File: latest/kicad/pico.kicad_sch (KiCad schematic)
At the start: 69 parts, among them J1 Jack 3.5mm, J12 Debug, J14 JST PH 4, J2 DIN5, J25 JST PH 3, J26 JST PH 3, J3 Jack 3.5mm, J4 DIN5, J5 Jack 6.35mm, J8 Jack 6.35mm, SW1 24P/R 24mm, SW10 Tactile Button, SW2 24P/R 24mm, SW3 Micro Button, SW4 Micro Button, SW5 Tactile Button, SW6 Tactile Button, SW7 Tactile Button, SW8 Tactile Button, SW9 Tactile Button, U12 AT24CS01-STUM, U2 TLP2761, U3 RP2040, U4 W25Q128JVS, Y2 ABM8-272-T3

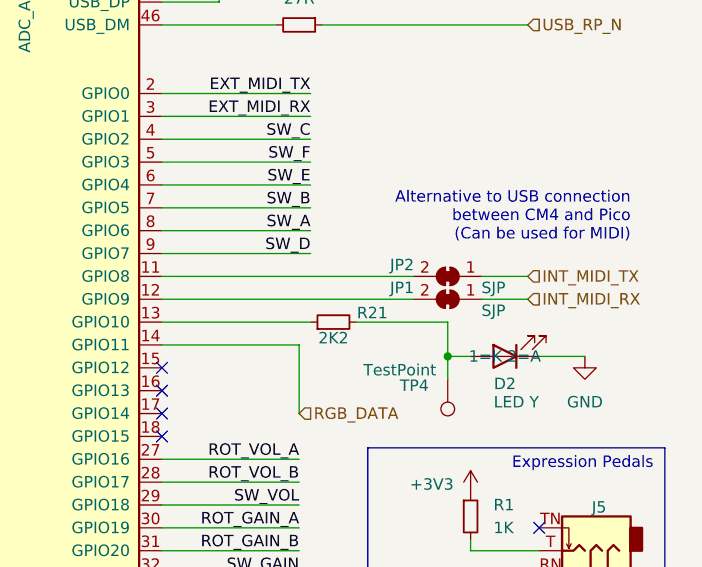
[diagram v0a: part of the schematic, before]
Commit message: Deploying to gh-pages from @ pedalboard/pedalboard-hw@99058ce3b2bc7db122aa04b2066b6492c6121c5a 🚀
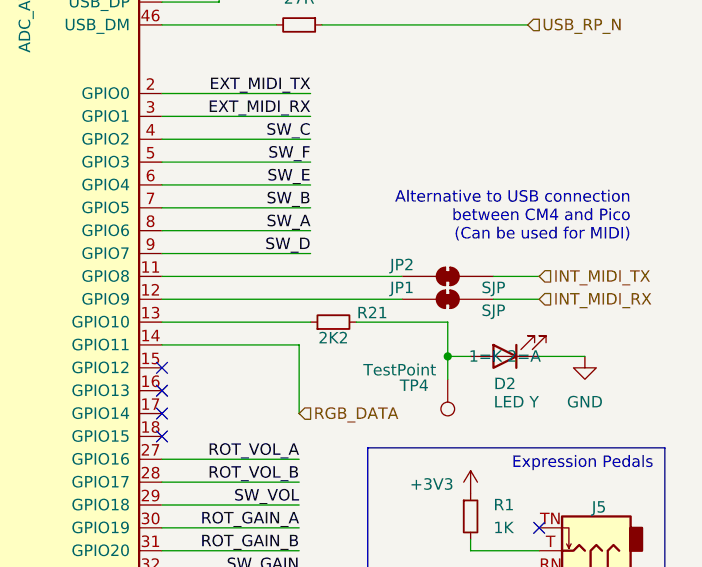
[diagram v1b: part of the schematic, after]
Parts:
- JP1, JP2: footprint Jumper:SolderJumper-2_P1.3mm_Bridged_RoundedPad1.0x1.5mm -> (none)
